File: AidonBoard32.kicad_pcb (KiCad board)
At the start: 2 copper layers, 49 x 63.3 mm, 33 parts, among them J1 RJ12, M1 MICRO_USB_18_TH, Q1 S8050, Q2 S8050, U1 AMS1117-3V3, U2 CP2102N-GQFN24, U3 ESP32-WROOM, U4 74HC04D

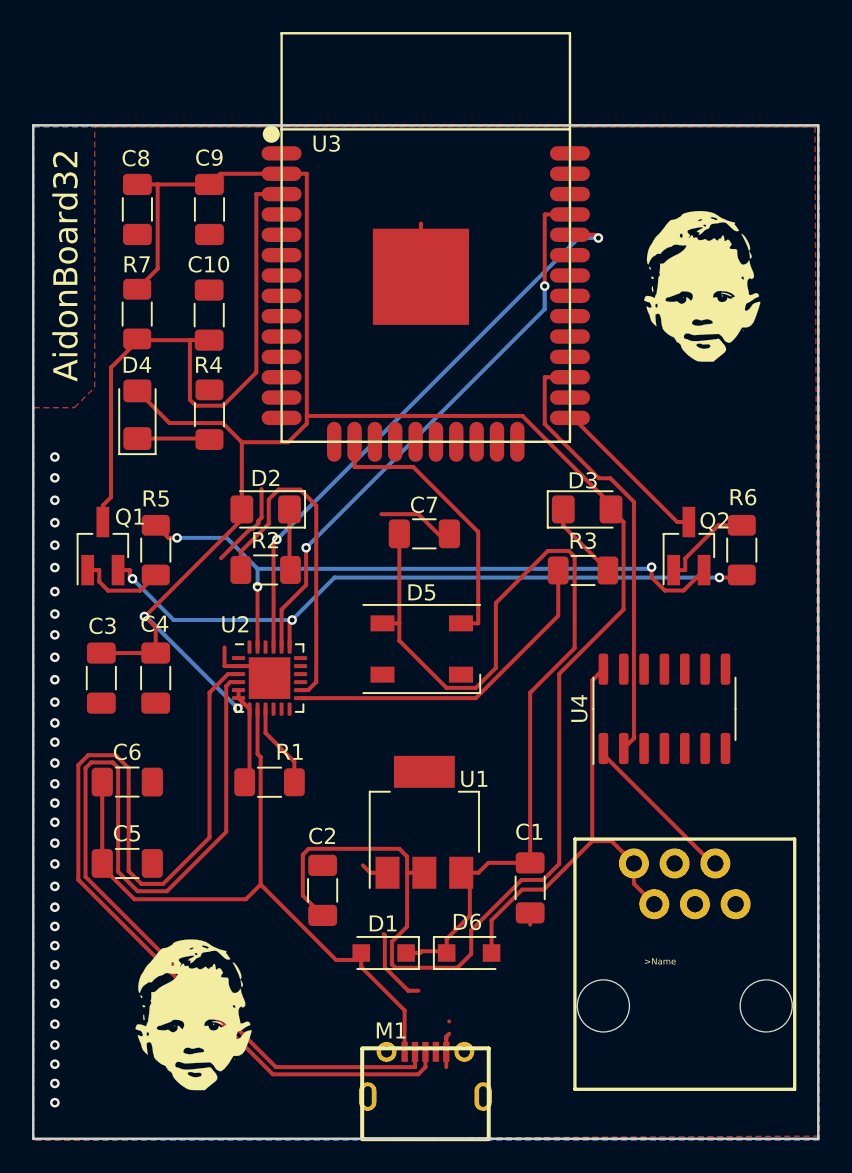
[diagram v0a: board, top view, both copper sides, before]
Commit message: Update
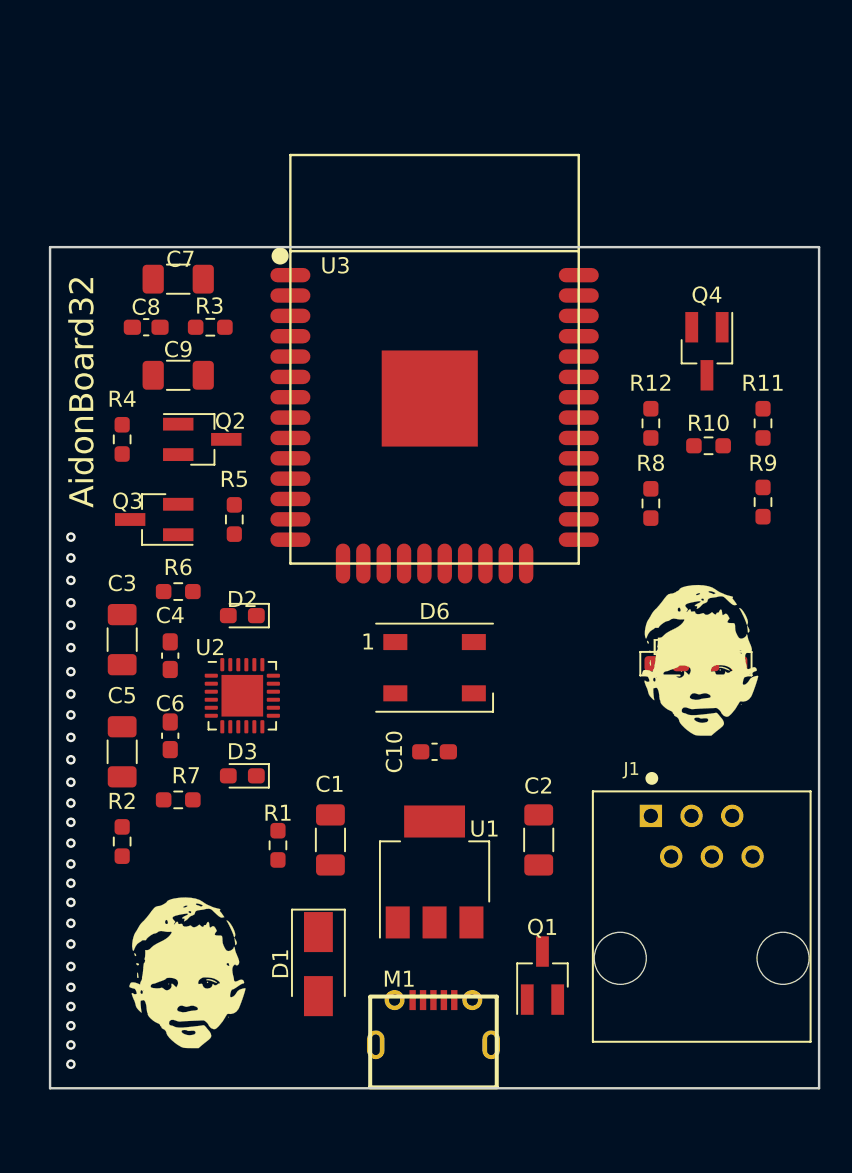
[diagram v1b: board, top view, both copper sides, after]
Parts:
- removed U4: 74HC04D, Package_SO:SOIC-14_3.9x8.7mm_P1.27mm
- added Q3: MMBT3904, Package_TO_SOT_SMD:SOT-23_Handsoldering, F.Cu at (85.5, 56.0)
- added Q4: MMBT3904, Package_TO_SOT_SMD:SOT-23_Handsoldering, F.Cu at (120.0, 45.5)
- added R10: 10K, Resistor_SMD:R_0603_1608Metric_Pad0.98x0.95mm_HandSolder, F.Cu at (120.1, 51.4)
- added R11: 1K, Resistor_SMD:R_0603_1608Metric_Pad0.98x0.95mm_HandSolder, F.Cu at (123.5, 50.0)
- added R12: 10K, Resistor_SMD:R_0603_1608Metric_Pad0.98x0.95mm_HandSolder, F.Cu at (116.5, 50.0)
- added R8: 220, Resistor_SMD:R_0603_1608Metric_Pad0.98x0.95mm_HandSolder, F.Cu at (116.5, 55.0)
- added R9: 220, Resistor_SMD:R_0603_1608Metric_Pad0.98x0.95mm_HandSolder, F.Cu at (123.5, 54.9)
- C10: value 10uF -> 0.1uF; footprint Capacitor_SMD:C_1206_3216Metric_Pad1.33x1.80mm_HandSolder -> Capacitor_SMD:C_0603_1608Metric_Pad1.08x0.95mm_HandSolder
- C4, C6: footprint Capacitor_SMD:C_1206_3216Metric_Pad1.33x1.80mm_HandSolder -> Capacitor_SMD:C_0603_1608Metric_Pad1.08x0.95mm_HandSolder
- C7: value 0.1uF -> 10uF
- C8: value 47uF -> 0.1uF; footprint Capacitor_SMD:C_1206_3216Metric_Pad1.33x1.80mm_HandSolder -> Capacitor_SMD:C_0603_1608Metric_Pad1.08x0.95mm_HandSolder
- C9: value 0.1uF -> 1uF
- D1: value 1N5819 -> SS54; footprint Diode_SMD:D_SOD-123F -> Diode_SMD:D_SMA
- D2, D3, D4: footprint LED_SMD:LED_1206_3216Metric_Pad1.42x1.75mm_HandSolder -> LED_SMD:LED_0603_1608Metric_Pad1.05x0.95mm_HandSolder
- D5: value WS2812B -> LED_Small; footprint LED_SMD:LED_WS2812B_PLCC4_5.0x5.0mm_P3.2mm -> LED_SMD:LED_0603_1608Metric_Pad1.05x0.95mm_HandSolder
- D6: value 1N5819 -> WS2812B; footprint Diode_SMD:D_SOD-123F -> LED_SMD:LED_WS2812B_PLCC4_5.0x5.0mm_P3.2mm
- J1: footprint Henrik-Connectors:RJ11-6 -> 5555165-1:TE_5555165-1
- M1: value MICRO_USB_18_TH -> U-F-M5DD-Y-L
- Q1: value S8050 -> Si2301CDS-T1-GE3
- Q2: value S8050 -> MMBT3904
- R1: value 1k -> 100K; footprint Resistor_SMD:R_1206_3216Metric_Pad1.30x1.75mm_HandSolder -> Resistor_SMD:R_0603_1608Metric_Pad0.98x0.95mm_HandSolder
- R2: value 1k -> 1K; footprint Resistor_SMD:R_1206_3216Metric_Pad1.30x1.75mm_HandSolder -> Resistor_SMD:R_0603_1608Metric_Pad0.98x0.95mm_HandSolder
- R3, R4: value 1k -> 10K; footprint Resistor_SMD:R_1206_3216Metric_Pad1.30x1.75mm_HandSolder -> Resistor_SMD:R_0603_1608Metric_Pad0.98x0.95mm_HandSolder
- R5: value 12k -> 10K; footprint Resistor_SMD:R_1206_3216Metric_Pad1.30x1.75mm_HandSolder -> Resistor_SMD:R_0603_1608Metric_Pad0.98x0.95mm_HandSolder
- R6: value 12k -> 220; footprint Resistor_SMD:R_1206_3216Metric_Pad1.30x1.75mm_HandSolder -> Resistor_SMD:R_0603_1608Metric_Pad0.98x0.95mm_HandSolder
- R7: value 1k -> 220; footprint Resistor_SMD:R_1206_3216Metric_Pad1.30x1.75mm_HandSolder -> Resistor_SMD:R_0603_1608Metric_Pad0.98x0.95mm_HandSolder
- moved Q1 38.4 mm to (109.7, 84.5)
- moved D4 36.5 mm to (117.5, 65.0), turned to 0 degrees
- moved R6 35.3 mm to (87.0, 60.5), turned to 180 degrees
- moved Q2 31.1 mm to (88.5, 51.0), turned to 0 degrees
- moved C10 30.7 mm to (103.0, 70.5), turned to 180 degrees
- moved R7 30.4 mm to (87.0, 73.5), turned to 180 degrees
- moved R3 27.8 mm to (89.0, 44.0)
- moved D3 27.2 mm to (91.0, 72.0), turned to 180 degrees
- moved G2 23.3 mm to (119.5, 65.0)
- moved C7 22.1 mm to (87.0, 41.0)
- moved R2 19.2 mm to (83.5, 76.1), turned to 270 degrees
- moved D5 18.9 mm to (121.1, 65.0), turned to 180 degrees
- moved D6 17.9 mm to (103.0, 65.2)
- moved C2 13.9 mm to (109.5, 76.0)
- moved C1 12.8 mm to (96.5, 76.0)
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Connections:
- C1 pad 1: +5V -> VCC
- C10 pad 1: /EN -> GND
- C10 pad 2: GND -> VCC
- C7 pad 1: GND -> +3V3
- C7 pad 2: +5V -> GND
- C9 pad 1: +3V3 -> /EN
- D1 pad 1: +5V -> VCC
- D2 pad 2: +3V3 -> Net-(D2-Pad2)
- D3 pad 2: +3V3 -> Net-(D2-Pad2)
- D4 pad 2: +3V3 -> Net-(D2-Pad2)
- D5 pad 1: +5V -> Net-(D5-Pad1)
- D5 pad 2: Net-(D5-Pad2) -> Net-(D2-Pad2)
- D6 pad 1: +5V -> VCC
- D6 pad 2: VDD -> Net-(D6-Pad2)
- J1 pad 1: VDD -> +5V
- J1 pad 2: VDD -> +5V
- J1 pad 3: Net-(J1-Pad3) -> GND
- Q1 pad 1: Net-(Q1-Pad1) -> VBUS
- Q1 pad 2: /RTS -> VCC
- Q1 pad 3: /EN -> +5V
- Q2 pad 2: /DTR -> /RTS
- Q2 pad 3: /IO0 -> /EN
- R1 pad 1: Net-(R1-Pad1) -> VBUS
- R1 pad 2: +3V3 -> GND
- R2 pad 1: /LED_TX -> Net-(R2-Pad1)
- R2 pad 2: Net-(D2-Pad1) -> +3V3
- R3 pad 1: /LED_RX -> +3V3
- R3 pad 2: Net-(D3-Pad1) -> /EN
- R4 pad 1: GND -> Net-(Q2-Pad1)
- R4 pad 2: Net-(D4-Pad1) -> /DTR
- R5 pad 1: Net-(Q1-Pad1) -> Net-(Q3-Pad1)
- R5 pad 2: /DTR -> /RTS
- R6 pad 1: Net-(Q2-Pad1) -> /LED_TX
- R6 pad 2: /RTS -> Net-(D2-Pad1)
- R7 pad 1: +3V3 -> /LED_RX
- R7 pad 2: /EN -> Net-(D3-Pad1)
- U1 pad 3: +5V -> VCC
- U2 pad 9: Net-(R1-Pad1) -> Net-(R2-Pad1)
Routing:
- net +3V3: track 159.2 -> 0.00 mm, vias 2 -> 0
- net /D+: track 63.1 -> 0.00 mm
- net /D-: track 60.8 -> 0.00 mm
- net +5V: track 59.0 -> 0.00 mm
- net /RTS: track 43.4 -> 0.00 mm, vias 3 -> 0
- net VBUS: track 43.0 -> 0.00 mm
- net /DTR: track 41.8 -> 0.00 mm, vias 3 -> 0
- net /EN: track 38.4 -> 0.00 mm
- net /MCU_RX: track 36.5 -> 0.00 mm, vias 2 -> 0
- net /MCU_TX: track 35.4 -> 0.00 mm, vias 2 -> 0
- net GND: track 28.2 -> 0.00 mm, vias 32 -> 25
- net /UART_RX: track 27.7 -> 0.00 mm
- net VDD: track 27.6 -> 0.00 mm
- net /LED_RX: track 21.0 -> 0.00 mm
- net /LED_TX: track 21.0 -> 0.00 mm
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- removed copper zone on B.Cu, net GND
- removed copper zone on F.Cu, net GND
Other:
- board size 49 x 63.3 mm -> 48 x 52.5 mm
